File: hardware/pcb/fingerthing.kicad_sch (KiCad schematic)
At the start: 46 parts, among them J1 10103594-0001LF, J2 TSW-118-07-L-D, J3 TSW-118-07-L-D, J4 SM03B-SRSS-TB(LF)(SN), SW1 434133025816, SW2 434133025816, U1 RP2350A, U2 NCP1117ST33T3G, U3 W25Q128JVSIQ, X1 12MHz

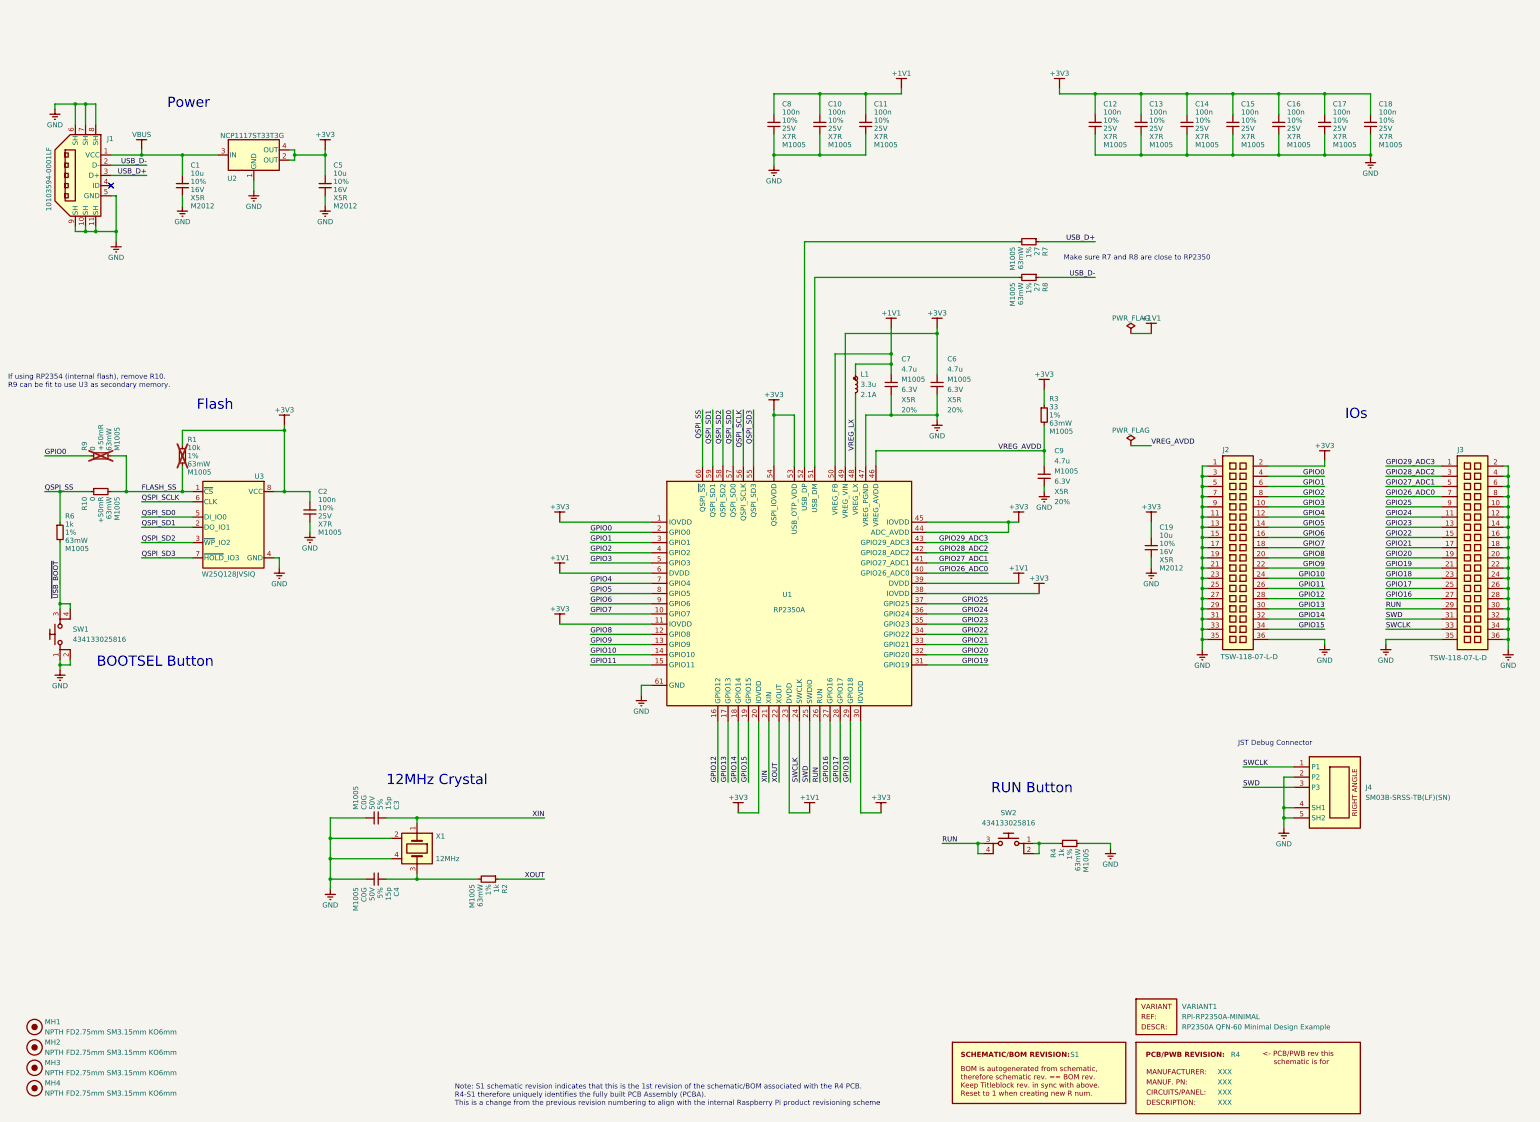
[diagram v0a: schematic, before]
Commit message: usb / sensor layout
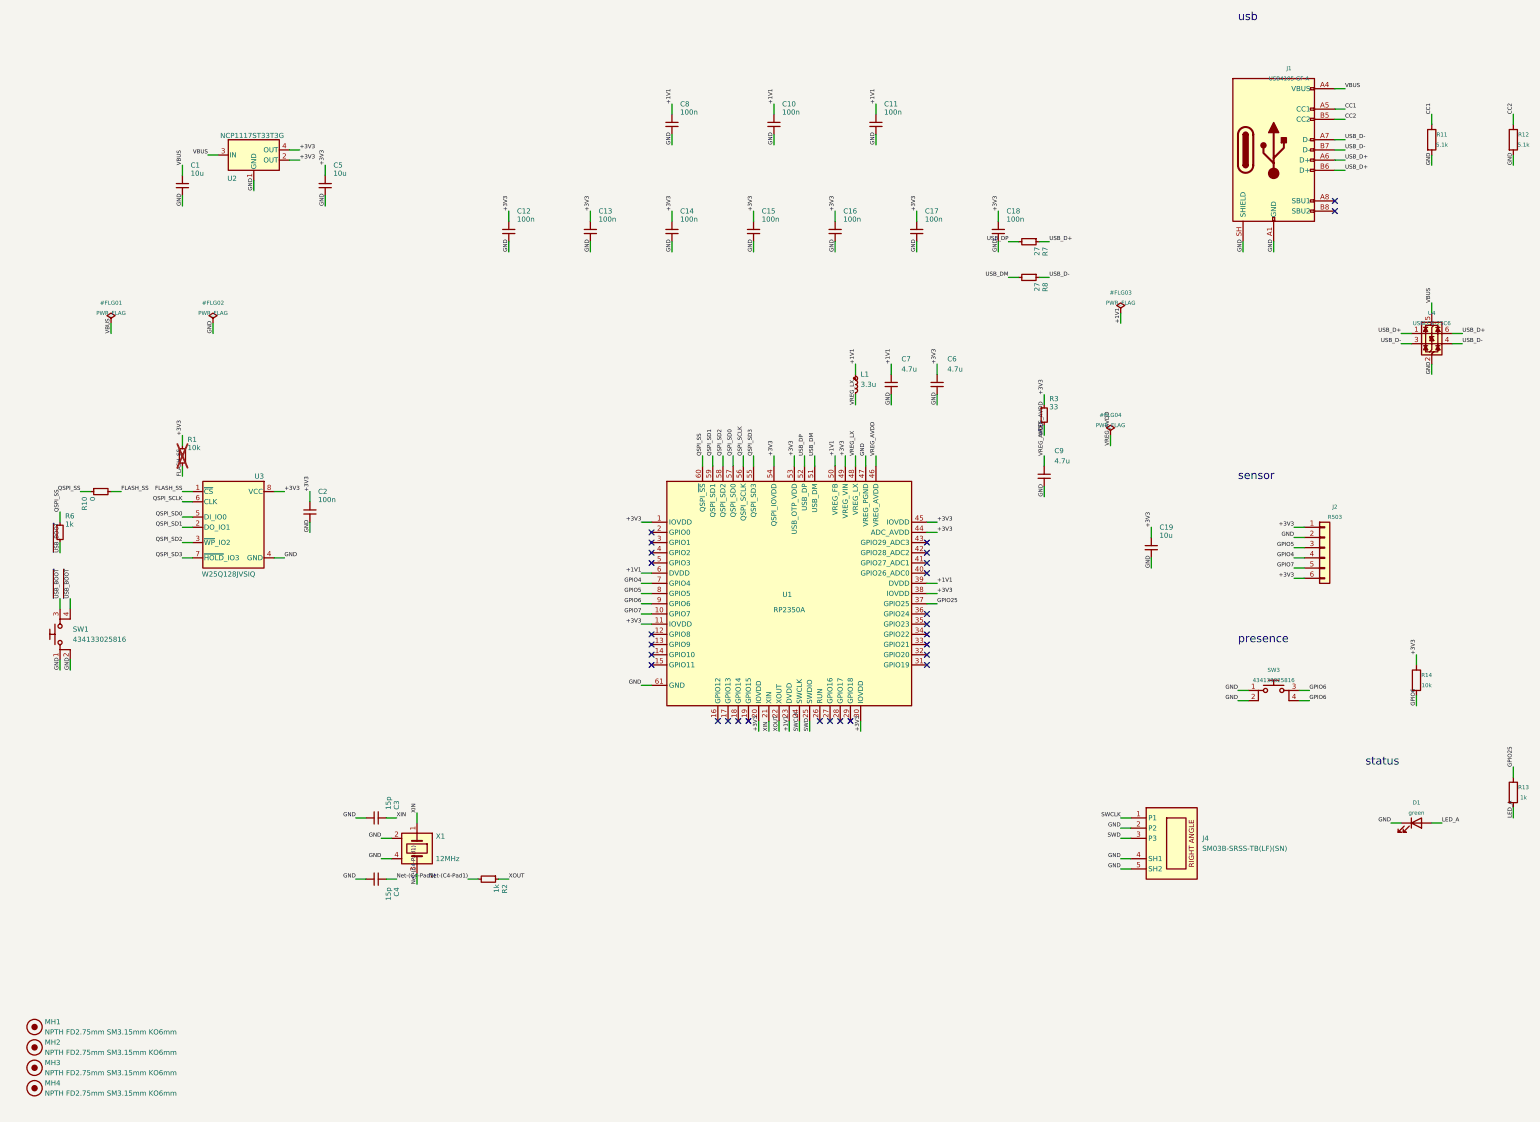
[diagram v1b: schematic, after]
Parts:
- removed J1: 10103594-0001LF, RPI_COMPILED:amphenol_10103594-0001lf, symbol fingerthing:RP-019A1P-1JAX7V
- removed J2, J3: TSW-118-07-L-D, RPI_COMPILED:samtec_tsw-118-07-l-d, symbol fingerthing:RP-01JWH2-G371Y4
- removed PCB1: R4, symbol fingerthing:PCB_PWB_REV
- removed R4: 1k, RPI_COMPILED:generic_resc1005x35, symbol fingerthing:RP-019A1P-4Z6ZWY
- removed R9: 0, RPI_COMPILED:generic_resc1005x35, symbol fingerthing:RP-019A1P-4Y4V63
- removed SBREV1: S1, symbol fingerthing:SCH_BOM_REV
- removed SW2: 434133025816, RPI_COMPILED:wurthelek_434133025816, symbol fingerthing:RP-01H0MT-6E9H8F
- removed VARIANT1: RPI-RP2350A-MINIMAL, symbol fingerthing:VARIANT
- added D1: green, LED_SMD:LED_0603_1608Metric, symbol Device:LED
- added J1: USB4105-GF-A, Connector_USB:USB_C_Receptacle_GCT_USB4105-xx-A_16P_TopMnt_Horizontal, symbol Connector:USB_C_Receptacle_USB2.0_16P
- added J2: R503, Connector_JST:JST_SH_SM06B-SRSS-TB_1x06-1MP_P1.00mm_Horizontal, symbol Connector_Generic:Conn_01x06
- added R11, R12: 5.1k, Resistor_SMD:R_0402_1005Metric, symbol Device:R
- added R13: 1k, Resistor_SMD:R_0402_1005Metric, symbol Device:R
- added R14: 10k, Resistor_SMD:R_0402_1005Metric, symbol Device:R
- added SW3: 434133025816, RPI_COMPILED:wurthelek_434133025816, symbol fingerthing:RP-01H0MT-6E9H8F
- added U4: USBLC6-2SC6, Package_TO_SOT_SMD:SOT-23-6, symbol Power_Protection:USBLC6-2SC6
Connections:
- net +3V3: now also J2.1 (Pin_1), J2.6 (Pin_6), R14.1
- net GND: now also D1.1 (K), J1.A1 (GND), J1.A12 (GND), J1.B1 (GND), J1.B12 (GND), J1.SH (SHIELD), J2.2 (Pin_2), R11.2, R12.2, SW3.1, SW3.2, U4.2 (GND)
- net GPIO25: now also R13.1
- net GPIO4: now also J2.4 (Pin_4)
- net GPIO5: now also J2.3 (Pin_3)
- net GPIO6: now also R14.2, SW3.3, SW3.4
- net GPIO7: now also J2.5 (Pin_5)
- net USB_D+: now also J1.A6 (D+), J1.B6 (D+), U4.1 (I/O1), U4.6 (I/O1)
- net USB_D-: now also J1.A7 (D-), J1.B7 (D-), U4.3 (I/O2), U4.4 (I/O2)
- net VBUS: now also J1.A4 (VBUS), J1.A9 (VBUS), J1.B4 (VBUS), J1.B9 (VBUS), U4.5 (VBUS)
- net USB_DP: now reaches R7.2, U1.52 (USB_DP)
- net USB_DM: now reaches R8.2, U1.51 (USB_DM)
- net Net-(C4-Pad1): now reaches C4.1, R2.2, X1.3
- net GPIO0: no longer names the net of U1.2 (GPIO0)
- net GPIO1: no longer names the net of U1.3 (GPIO1)
- net GPIO10: no longer names the net of U1.14 (GPIO10)
- net GPIO11: no longer names the net of U1.15 (GPIO11)
- net GPIO12: no longer names the net of U1.16 (GPIO12)
- net GPIO13: no longer names the net of U1.17 (GPIO13)
- net GPIO14: no longer names the net of U1.18 (GPIO14)
- net GPIO15: no longer names the net of U1.19 (GPIO15)
- net GPIO16: no longer names the net of U1.27 (GPIO16)
- net GPIO17: no longer names the net of U1.28 (GPIO17)
- net GPIO18: no longer names the net of U1.29 (GPIO18)
- net GPIO19: no longer names the net of U1.31 (GPIO19)
- net GPIO2: no longer names the net of U1.4 (GPIO2)
- net GPIO20: no longer names the net of U1.32 (GPIO20)
- net GPIO21: no longer names the net of U1.33 (GPIO21)
- net GPIO22: no longer names the net of U1.34 (GPIO22)
- net GPIO23: no longer names the net of U1.35 (GPIO23)
- net GPIO24: no longer names the net of U1.36 (GPIO24)
- net GPIO26_ADC0: no longer names the net of U1.40 (GPIO26_ADC0)
- net GPIO27_ADC1: no longer names the net of U1.41 (GPIO27_ADC1)
- net GPIO28_ADC2: no longer names the net of U1.42 (GPIO28_ADC2)
- net GPIO29_ADC3: no longer names the net of U1.43 (GPIO29_ADC3)
- net GPIO3: no longer names the net of U1.5 (GPIO3)
- net GPIO8: no longer names the net of U1.12 (GPIO8)
- net GPIO9: no longer names the net of U1.13 (GPIO9)
- net RUN: no longer names the net of U1.26 (RUN)
- new net CC1: J1.A5 (CC1), R11.1
- new net CC2: J1.B5 (CC2), R12.1
- new net LED_A: D1.2 (A), R13.2
- no-connect marks 1 -> 28
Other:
- note added: "presence"
- note added: "sensor"
- note added: "status"
- note added: "usb"
- note removed: "12MHz Crystal"
- note removed: "BOOTSEL Button"
- note removed: "Flash"
- note removed: "IOs"
- note removed: "If using RP2354 (internal flash), remove R10. R9 can be fit to use U3 as secondary memory."
- note removed: "JST Debug Connector"
- note removed: "Make sure R7 and R8 are close to RP2350"
- note removed: "Note: S1 schematic revision indicates that this is the 1st revision of the schematic/BOM associated with the R4 PCB. R4-S1 therefore uniquely identifies the fully built PCB Assembly (PCBA). This is a change from the previous revision numbering to align with the internal Raspberry Pi product revisioning scheme"
- note removed: "Power"
- note removed: "RUN Button"
- moved on the sheet: C10, C11, C12, C13, C14, C15, C16, C17, C18, C8, J4
